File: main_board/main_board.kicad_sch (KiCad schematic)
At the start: 0 parts

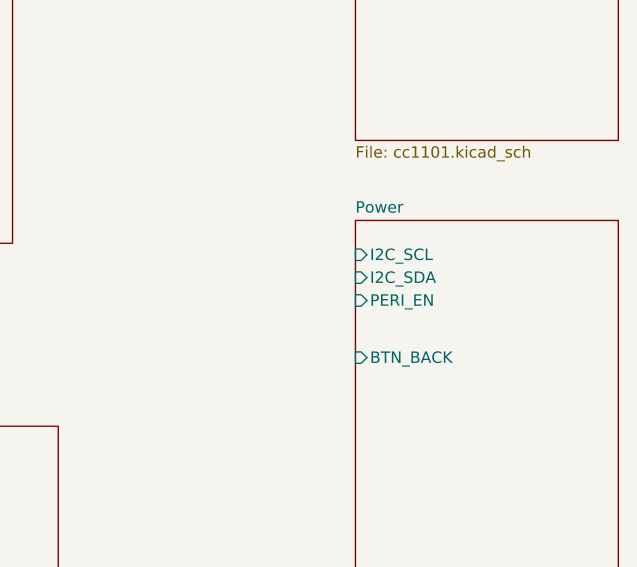
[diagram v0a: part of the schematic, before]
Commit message: sch: update sch
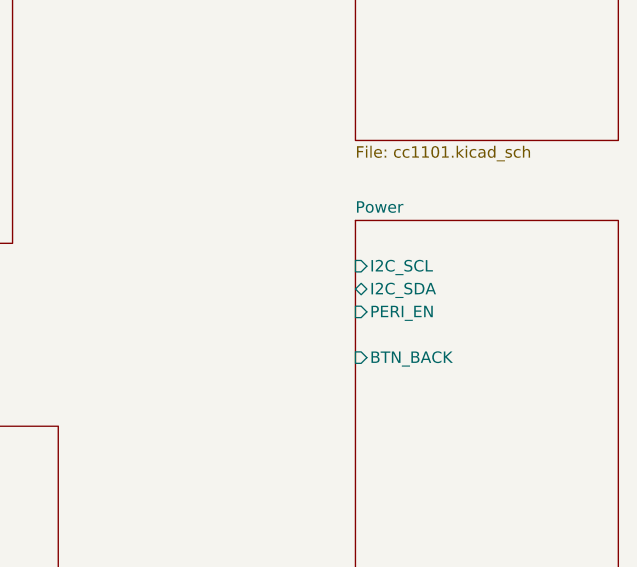
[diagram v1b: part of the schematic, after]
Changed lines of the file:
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@@
 			)
 		)
-		(pin "I2C_SDA" input
-			(at 204.47 125.73 180)
+		(pin "BTN_BACK" input
+			(at 204.47 134.62 180)
 			(effects
 				(font
@@
 		)
 		(pin "I2C_SCL" input
-			(at 204.47 123.19 180)
+			(at 204.47 124.46 180)
+			(effects
+				(font
+					(size 1.27 1.27)
+				)
+				(justify left)
+			)
+		)
+		(pin "I2C_SDA" bidirectional
+			(at 204.47 127 180)
 			(effects
 				(font
@@
 		)
 		(pin "PERI_EN" input
-			(at 204.47 128.27 180)
+			(at 204.47 129.54 180)
 			(effects
 				(font
-					(size 1.27 1.27)
-				)
-				(justify left)
-			)
-		)
-		(pin "BTN_BACK" input
-			(at 204.47 134.62 180)
-			(effects
-				(font
